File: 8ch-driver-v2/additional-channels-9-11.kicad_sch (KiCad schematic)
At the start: 42 parts, among them Q10 2N7002E, Q11 2N7002E, Q9 2N7002E, U10 DRV104PWP, U11 DRV104PWP, U9 DRV104PWP

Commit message: progress
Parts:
- U9: footprint Solenoid_Driver:IC_TPS27S100BPWPR -> Solenoid_Driver:PWP14_2P31X2P46
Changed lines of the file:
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@@
 			)
 		)
-		(property "Footprint" "Solenoid_Driver:IC_TPS27S100BPWPR"
+		(property "Footprint" "Solenoid_Driver:PWP14_2P31X2P46"
 			(at 147.32 45.72 0)
 			(effects

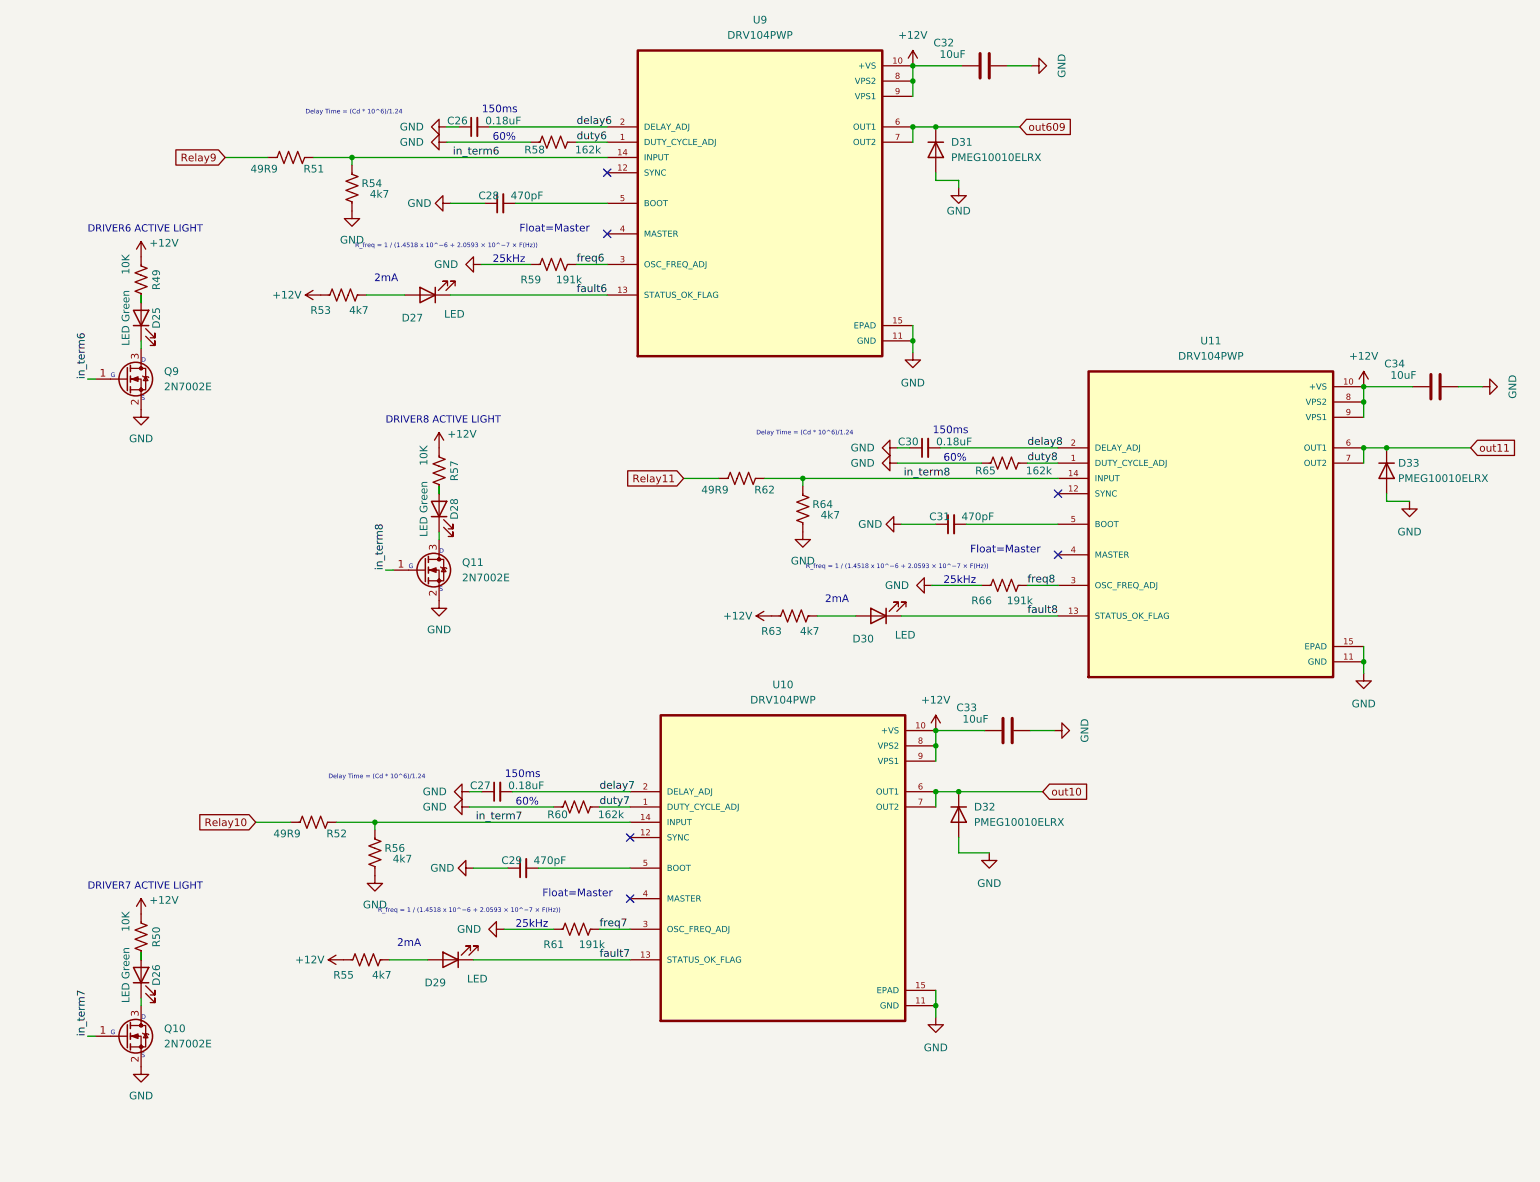
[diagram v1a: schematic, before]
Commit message: mucho mas progresso
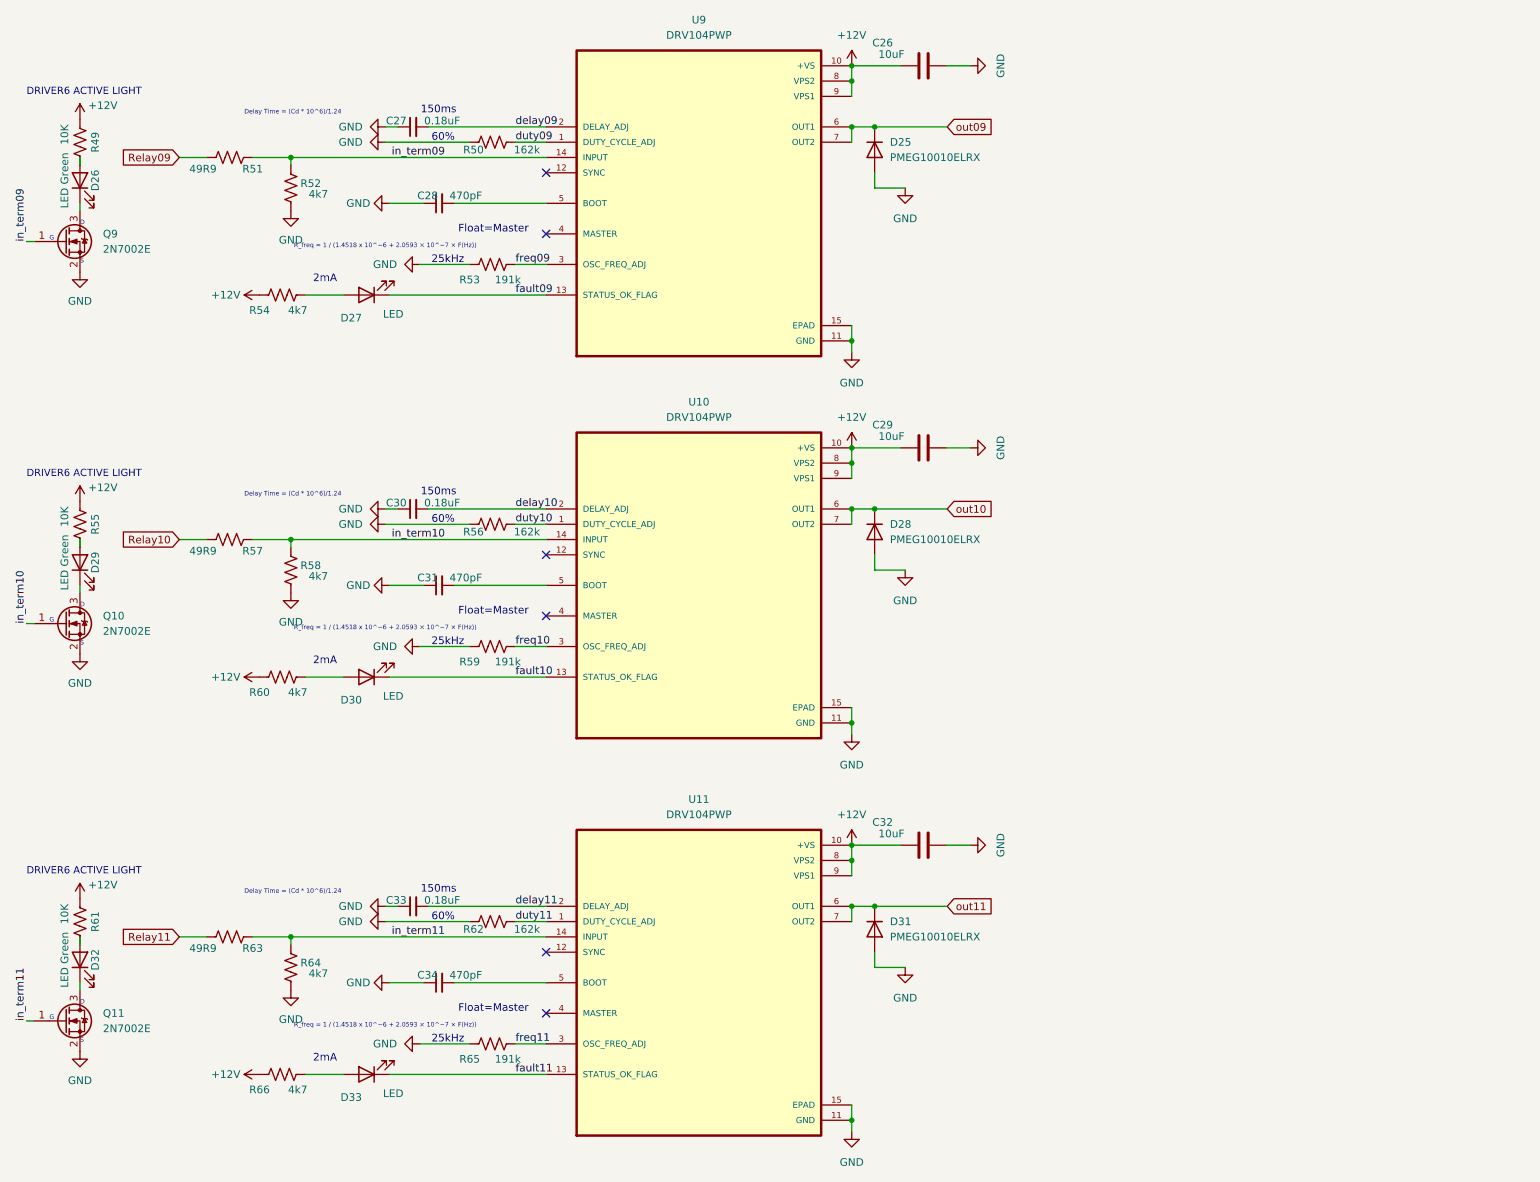
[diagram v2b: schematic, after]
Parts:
- removed C26: 0.18uF, Capacitor_SMD:C_1206_3216Metric, symbol Device:C_Small
- removed C29: 470pF, Capacitor_SMD:C_1206_3216Metric, symbol Device:C_Small
- removed C33, C34: 10uF, Capacitor_SMD:C_1210_3225Metric, symbol Device:C
- removed D25, D28: LED Green, LED_SMD:LED_0805_2012Metric, symbol Device:LED
- removed D32, D33: PMEG10010ELRX, Diode_SMD:Nexperia_CFP3_SOD-123W, symbol Device:D
- added C26, C29: 10uF, Capacitor_SMD:C_1210_3225Metric, symbol Device:C
- added C33: 0.18uF, Capacitor_SMD:C_1206_3216Metric, symbol Device:C_Small
- added C34: 470pF, Capacitor_SMD:C_1206_3216Metric, symbol Device:C_Small
- added D25, D28: PMEG10010ELRX, Diode_SMD:Nexperia_CFP3_SOD-123W, symbol Device:D
- added D32: LED Green, LED_SMD:LED_0805_2012Metric, symbol Device:LED
- added D33: LED, LED_SMD:LED_0805_2012Metric, symbol Device:LED
- D29: value LED -> LED Green
- R50: value 10K -> 162k
- R52: value 49R9 -> 4k7; PartNum RC0805FR-0749R9L -> RC0805JR-074K7L
- R53: value 4k7 -> 191k; PartNum RC0805JR-074K7L -> RC0805FR-07191KL
- R55: value 4k7 -> 10K; PartNum RC0805JR-074K7L -> RC0805FR-07162KL
- R56: value 4k7 -> 162k; PartNum RC0805JR-074K7L -> RC0805FR-07162KL
- R57: value 10K -> 49R9; PartNum RC0805FR-07162KL -> RC0805FR-0749R9L
- R58, R60: value 162k -> 4k7; PartNum RC0805FR-07162KL -> RC0805JR-074K7L
- R61: value 191k -> 10K; PartNum RC0805FR-07191KL -> RC0805FR-07162KL
- R62: value 49R9 -> 162k; PartNum RC0805FR-0749R9L -> RC0805FR-07162KL
- R63: value 4k7 -> 49R9; PartNum RC0805JR-074K7L -> RC0805FR-0749R9L
- R65: value 162k -> 191k; PartNum RC0805FR-07162KL -> RC0805FR-07191KL
- R66: value 191k -> 4k7; PartNum RC0805FR-07191KL -> RC0805JR-074K7L
- U9: footprint Solenoid_Driver:PWP14_2P31X2P46 -> Solenoid_Driver:IC_TPS27S100BPWPR
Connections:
- net +12V: now also R54.1, R60.1, R61.1, R66.1, C26.1, C29.1; no longer R50.1, R53.1, R57.1, R63.1
- net GND: now also R50.1, R52.1, R53.1, R62.1, C26.2, C29.2, C33.1, C34.1, D25.2 (A), D28.2 (A); no longer R54.1, R60.1, R61.1, R66.1
- net Relay10: now also R57.1; no longer R52.1
- net Relay11: now also R63.1; no longer R62.1
- net out10: now also D28.1 (K)
- net out11: now also D31.1 (K)
- net at D27.2 (A): now also R54.2; no longer R53.2
- net at D26.2 (A): now also R49.2; no longer R50.2
- net at Q9.3 (D): now also D26.1 (K)
- net at C31.2: now also U10.5 (BOOT); no longer U11.5 (BOOT)
- net at Q11.3 (D): now also D32.1 (K)
- net at D30.2 (A): now also R60.2; no longer R63.2
- net in_term10: now reaches R57.2
- net in_term10: now also Q10.1 (G), R58.2, U10.14 (INPUT)
- net at Q10.3 (D): now also D29.1 (K); no longer D26.1 (K)
- net Relay9 renamed Relay09
- net delay6 renamed delay09
- net delay09: now also C27.2
- net delay7 renamed delay10
- net delay10: now also C30.2; no longer C27.2
- net delay8 renamed delay11
- net delay11: now also C33.2; no longer C30.2
- net duty6 renamed duty09
- net duty09: now also R50.2; no longer R58.2
- net duty7 renamed duty10
- net duty10: now also R56.2; no longer R60.2
- net duty8 renamed duty11
- net duty11: now also R62.2; no longer R65.2
- net fault6 renamed fault09
- net fault7 renamed fault10
- net fault10: now also D30.1 (K); no longer D29.1 (K)
- net fault8 renamed fault11
- net fault11: now also D33.1 (K); no longer D30.1 (K)
- net freq6 renamed freq09
- net freq09: now also R53.2; no longer R59.2
- net freq7: no longer names the net of R61.2
- net freq7: now also D32.2 (A); no longer U10.3 (OSC_FREQ_ADJ)
- net freq8: no longer names the net of R66.2
- net freq8: now also D33.2 (A); no longer U11.3 (OSC_FREQ_ADJ)
- net in_term6 renamed in_term09
- net in_term09: now also R52.2; no longer R54.2
- removed net in_term7: Q10.1 (G), R52.2, R56.2, U10.14 (INPUT)
- net in_term8 renamed in_term11
- net in_term11: now also R63.2; no longer R62.2
- net out609 renamed out09
- net out09: now also D25.1 (K); no longer D31.1 (K)
- new net: C34.2, U11.5 (BOOT)
- new net freq10: R59.2, U10.3 (OSC_FREQ_ADJ)
- new net freq11: R65.2, U11.3 (OSC_FREQ_ADJ)
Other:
- note removed: "DRIVER7 ACTIVE LIGHT"
- note removed: "DRIVER8 ACTIVE LIGHT"
